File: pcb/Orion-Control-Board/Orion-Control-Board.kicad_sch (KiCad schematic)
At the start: 59 parts, among them J1 CONN_20_POS_KEYED_SOCKET, U1 BNO055, U2 INA3221, U3 DFR0753 5V BUCK, U4 PCA9685_PWM_SERVO_DRIVER_IC, U5 INA3221, U6 INA3221, Y1 32.768 kHz

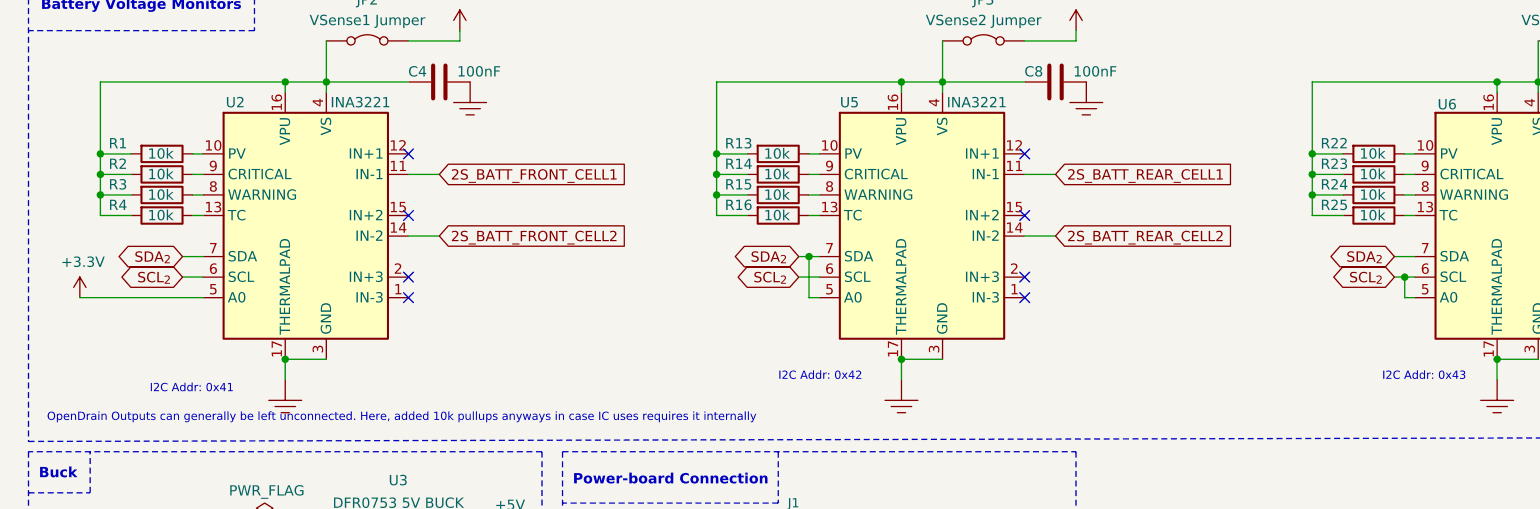
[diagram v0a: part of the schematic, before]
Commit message: Route more
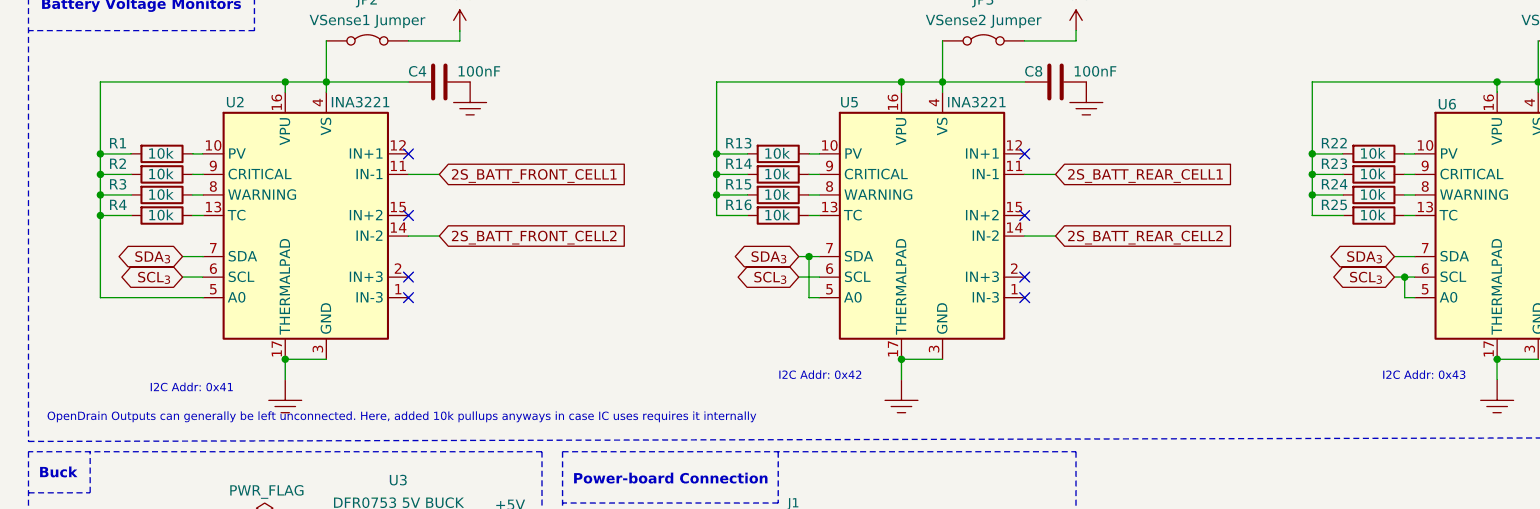
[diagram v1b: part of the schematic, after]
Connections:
- net SCL_{2} is gone; now on net SCL_{3}: U2.6 (SCL), U5.6 (SCL), U6.5 (A0), U6.6 (SCL)
- net SDA_{2} is gone; now on net SDA_{3}: U2.7 (SDA), U5.5 (A0), U5.7 (SDA), U6.7 (SDA)
- net +3.3V: no longer U2.5 (A0)
- net at C4.1, JP2.1 (A), R1.2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: now also U2.5 (A0)
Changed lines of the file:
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@@
 	)
 	(junction
+		(at 24.13 132.08)
+		(diameter 0)
+		(color 0 0 0 0)
+	)
+	(junction
 		(at 100.33 129.54)
 		(diameter 0)
@@
 	(wire
 		(pts
+			(xy 24.13 142.24) (xy 36.83 142.24)
+		)
+		(stroke
+			(width 0)
+			(type default)
+		)
+	)
+	(wire
+		(pts
 			(xy 185.42 139.7) (xy 186.69 139.7)
 		)
@@
 	(wire
 		(pts
+			(xy 24.13 142.24) (xy 24.13 132.08)
+		)
+		(stroke
+			(width 0)
+			(type default)
+		)
+	)
+	(wire
+		(pts
 			(xy 224.79 39.37) (xy 228.6 39.37)
 		)
@@
 	(wire
 		(pts
-			(xy 21.59 142.24) (xy 36.83 142.24)
-		)
-		(stroke
-			(width 0)
-			(type default)
-		)
-	)
-	(wire
-		(pts
 			(xy 45.72 86.36) (xy 46.99 86.36)
 		)
@@
 		)
 	)
-	(global_label "SCL_{2}"
+	(global_label "SCL_{3}"
 		(shape bidirectional)
 		(at 110.49 139.7 180)
@@
 		)
 	)
-	(global_label "SDA_{2}"
+	(global_label "SDA_{3}"
 		(shape bidirectional)
 		(at 110.49 137.16 180)
@@
 		)
 	)
-	(global_label "SCL_{2}"
+	(global_label "SCL_{3}"
 		(shape bidirectional)
 		(at 184.15 139.7 180)
@@
 		)
 	)
-	(global_label "SDA_{2}"
+	(global_label "SDA_{3}"
 		(shape bidirectional)
 		(at 34.29 137.16 180)
@@
 		)
 	)
-	(global_label "SDA_{2}"
+	(global_label "SDA_{3}"
 		(shape bidirectional)
 		(at 184.15 137.16 180)
@@
 		)
 	)
-	(global_label "SCL_{2}"
+	(global_label "SCL_{3}"
 		(shape bidirectional)
 		(at 34.29 139.7 180)
@@
 					(unit 1)
 				)
-			)
-		)
-	)
-	(symbol
-		(lib_id "power:+3.3V")
-		(at 21.59 142.24 0)
-		(unit 1)
-		(exclude_from_sim no)
-		(in_bom yes)
-		(on_board yes)
-		(dnp no)
-		(property "Reference" "#PWR02"
-			(at 21.59 146.05 0)
-			(effects
-				(font
-					(size 1.27 1.27)
-				)
-				(hide yes)
-			)
-		)
-		(property "Value" "+3.3V"
-			(at 21.971 137.8458 0)
-			(effects
-				(font
-					(size 1.27 1.27)
-				)
-			)
-		)
-		(property "Footprint" ""
-			(at 21.59 142.24 0)
-			(effects
-				(font
-					(size 1.27 1.27)
-				)
-				(hide yes)
-			)
-		)
-		(property "Datasheet" ""
-			(at 21.59 142.24 0)
-			(effects
-				(font
-					(size 1.27 1.27)
-				)
-				(hide yes)
-			)
-		)
-		(property "Description" "Power symbol creates a global label with name \"+3.3V\""
-			(at 21.59 142.24 0)
-			(effects
-				(font
-					(size 1.27 1.27)
-				)
-				(hide yes)
-			)
-		)
-		(pin "1"
-		)
-		(instances
-			(project "Orion-Control-Board"
-				(path "/0755aee5-bc01-4cb5-b830-583289df50a3"
-					(reference "#PWR02")
-					(unit 1)
-				)
